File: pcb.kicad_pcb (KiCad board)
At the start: 2 copper layers, 40.6 x 40.6 mm, 3 parts

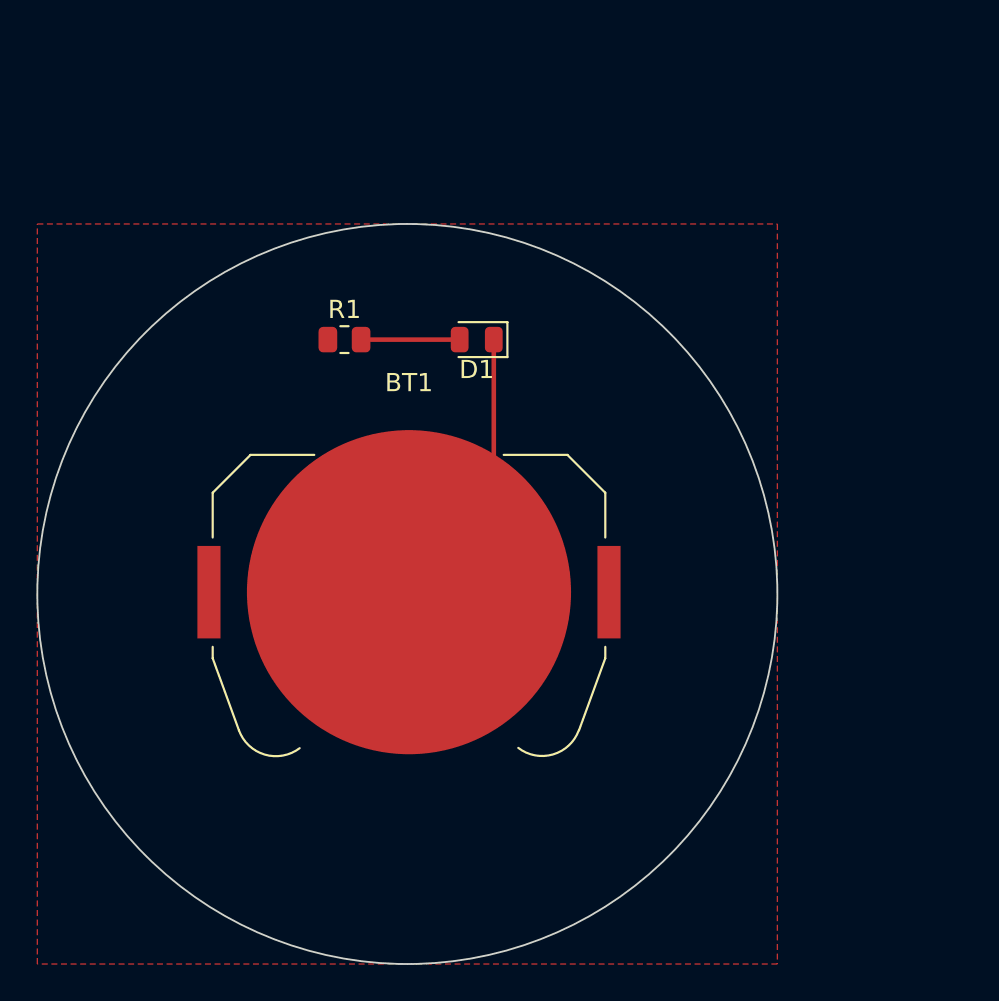
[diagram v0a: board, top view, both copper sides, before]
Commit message: inital layout
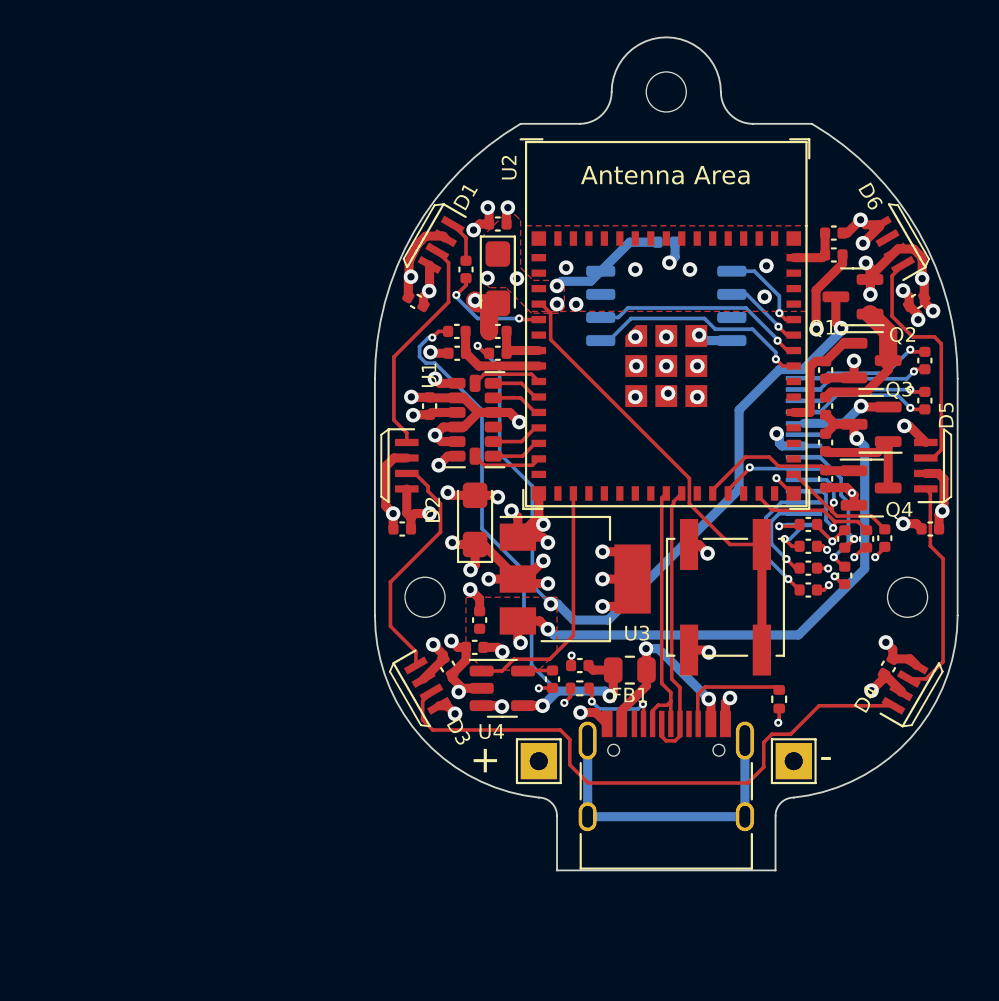
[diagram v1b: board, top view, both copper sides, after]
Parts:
- removed BT1: CR2032, Battery:BatteryHolder_Keystone_3034_1x20mm
- added C1: 100n, Capacitor_SMD:C_0402_1005Metric, F.Cu at (145.2, 67.8)
- added C10: 100n, Capacitor_SMD:C_0402_1005Metric, F.Cu at (146.0, 73.5)
- added C11: 4u7, Capacitor_SMD:C_0402_1005Metric, F.Cu at (154.2, 87.8)
- added C12: 4u7, Capacitor_SMD:C_0402_1005Metric, F.Cu at (168.8, 80.8)
- added C13: 100n, Capacitor_SMD:C_0402_1005Metric, F.Cu at (168.8, 82.8)
- added C14: 1u, Capacitor_SMD:C_0402_1005Metric, F.Cu at (173.2, 73.2)
- added C15: 2u2, Capacitor_SMD:C_0402_1005Metric, F.Cu at (166.8, 82.4)
- added C16: 4u7, Capacitor_SMD:C_0402_1005Metric, F.Cu at (166.8, 81.2)
- added C17: 1u, Capacitor_SMD:C_0402_1005Metric, F.Cu at (173.2, 71.0)
- added C18: 100n, Capacitor_SMD:C_0402_1005Metric, F.Cu at (166.8, 80.0)
- added C19: 1u, Capacitor_SMD:C_0402_1005Metric, F.Cu at (168.2, 64.0)
- added C2: 100n, Capacitor_SMD:C_0402_1005Metric, F.Cu at (144.5, 80.2)
- added C20: 10u tantalum, Capacitor_Tantalum_SMD:CP_EIA-3216-10_Kemet-I, F.Cu at (149.8, 66.5)
- added C21: 100n, Capacitor_SMD:C_0402_1005Metric, F.Cu at (149.8, 63.5)
- added C22: 100n, Capacitor_SMD:C_0402_1005Metric, B.Cu at (159.0, 64.5)
- added C3: 100n, Capacitor_SMD:C_0402_1005Metric, F.Cu at (147.0, 87.8)
- added C4: 100n, Capacitor_SMD:C_0402_1005Metric, F.Cu at (171.2, 87.8)
- added C5: 100n, Capacitor_SMD:C_0402_1005Metric, F.Cu at (173.5, 80.2)
- added C6: 100n, Capacitor_SMD:C_0402_1005Metric, F.Cu at (172.8, 67.8)
- added C7: 10u, Capacitor_SMD:C_0402_1005Metric, F.Cu at (148.8, 85.2)
- added C8: 10u tantalum, Capacitor_Tantalum_SMD:CP_EIA-3216-10_Kemet-I, F.Cu at (148.5, 79.8)
- added C9: 100n, Capacitor_SMD:C_0402_1005Metric, F.Cu at (148.5, 86.8)
- added D2: WS2812B-4020, WS2812B-4020:WS2812B-4020, F.Cu at (144.8, 76.8)
- added D3: WS2812B-4020, WS2812B-4020:WS2812B-4020, F.Cu at (145.9, 88.9)
- added D4: WS2812B-4020, WS2812B-4020:WS2812B-4020, F.Cu at (172.1, 88.9)
- added D5: WS2812B-4020, WS2812B-4020:WS2812B-4020, F.Cu at (173.2, 76.8)
- added D6: WS2812B-4020, WS2812B-4020:WS2812B-4020, F.Cu at (171.4, 64.6)
- added FB1: 100R@100MHz, Resistor_SMD:R_0805_2012Metric, F.Cu at (157.0, 88.0)
- added H1: MountingHole, MountingHole:MountingHole_2.2mm_M2, F.Cu at (172.2, 84.0)
- added H2: MountingHole, MountingHole:MountingHole_2.2mm_M2, F.Cu at (145.8, 84.0)
- added H3: MountingHole, MountingHole:MountingHole_2.2mm_M2, F.Cu at (159.0, 56.2)
- added J1: USB_C_Receptacle_USB2.0, Connector_USB:USB_C_Receptacle_HRO_TYPE-C-31-M-12, F.Cu at (159.0, 95.0)
- added J2: OLED, OLED_FFC:FPC_14, B.Cu at (166.6, 76.0)
- added Q1: 2N7002, Package_TO_SOT_SMD:SOT-23, F.Cu at (170.2, 71.0)
- added Q2: Si2301CDS, Package_TO_SOT_SMD:SOT-23, F.Cu at (169.2, 67.5)
- added Q3: 2N7002, Package_TO_SOT_SMD:SOT-23, F.Cu at (170.2, 78.0)
- added Q4: Si2301CDS, Package_TO_SOT_SMD:SOT-23, F.Cu at (170.2, 74.5)
- added R10: 4k7, Capacitor_SMD:C_0402_1005Metric, F.Cu at (170.0, 80.8)
- added R11: 4k7, Capacitor_SMD:C_0402_1005Metric, F.Cu at (171.0, 80.8)
- added R12: 10k, Capacitor_SMD:C_0402_1005Metric, F.Cu at (168.2, 65.2)
- added R15: 100k, Capacitor_SMD:C_0402_1005Metric, F.Cu at (149.8, 70.6)
- added R16: 100k, Capacitor_SMD:C_0402_1005Metric, F.Cu at (149.8, 69.4)
- added R17: 100k, Capacitor_SMD:C_0402_1005Metric, F.Cu at (147.5, 69.4)
- added R18: 100k, Capacitor_SMD:C_0402_1005Metric, F.Cu at (147.5, 70.6)
- added R2: 10k, Capacitor_SMD:C_0402_1005Metric, F.Cu at (167.8, 73.5)
- added R3: 10k, Capacitor_SMD:C_0402_1005Metric, F.Cu at (167.8, 77.5)
- added R4: 100, Capacitor_SMD:C_0402_1005Metric, F.Cu at (148.0, 66.0)
- added R5: 10k, Capacitor_SMD:C_0402_1005Metric, F.Cu at (152.8, 88.5)
- added R6: 5k1, Resistor_SMD:R_0402_1005Metric, F.Cu at (154.2, 89.0)
- added R7: 5k1, Resistor_SMD:R_0402_1005Metric, F.Cu at (165.2, 89.6)
- added R8: 10k, Capacitor_SMD:C_0402_1005Metric, F.Cu at (167.8, 75.5)
- added R9: 560k, Capacitor_SMD:C_0402_1005Metric, F.Cu at (166.8, 83.6)
- added SW1: SW_Push, Button_Switch_SMD:SW_Push_1P1T_NO_CK_KSC7xxJ, F.Cu at (162.2, 84.0)
- added TP1: Batt+, TestPoint:TestPoint_THTPad_2.0x2.0mm_Drill1.0mm, F.Cu at (152.0, 93.0)
- added TP2: Batt-, TestPoint:TestPoint_THTPad_2.0x2.0mm_Drill1.0mm, F.Cu at (166.0, 93.0)
- added U1: ADXL375, Package_LGA:LGA-14_3x5mm_P0.8mm_LayoutBorder1x6y, F.Cu at (148.5, 74.2)
- added U2: ESP32-S3-MINI-1, PCM_Espressif:ESP32-S2-MINI-1, F.Cu at (159.0, 71.3)
- added U3: AMS1117-3.3, Package_TO_SOT_SMD:SOT-223-3_TabPin2, F.Cu at (154.0, 83.0)
- added U4: MCP73831-2-OT, Package_TO_SOT_SMD:SOT-23-5, F.Cu at (150.0, 89.0)
- added U5: W25Q128JVS, Package_SO:SOIC-8_5.23x5.23mm_P1.27mm, B.Cu at (159.0, 68.0)
- D1: value LED -> WS2812B-4020; footprint LED_SMD:LED_0805_2012Metric -> WS2812B-4020:WS2812B-4020
- R1: value 1k -> 10k; footprint Resistor_SMD:R_0805_2012Metric -> Capacitor_SMD:C_0402_1005Metric
- moved R1 26.5 mm to (167.8, 71.5), turned to -90 degrees
- moved D1 5.56 mm to (146.6, 64.6), turned to 60 degrees
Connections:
- D1 pad 1: GND -> Net-(D1-DIN)
- D1 pad 2: Net-(D1-A) -> /LEDs/VLED
- R1 pad 1: Net-(BT1-+) -> LED_EN
- R1 pad 2: Net-(D1-A) -> GND
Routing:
- net VBAT: track 0.00 -> 86.6 mm, vias 0 -> 8
- net GND: track 15.6 -> 78.2 mm, vias 0 -> 58
- net +3.3V: track 0.00 -> 46.1 mm, vias 0 -> 21
- net USB_VBUS: track 0.00 -> 32.4 mm, vias 0 -> 3
- net Net-(D3-DOUT): track 0.00 -> 32.4 mm
- net /LEDs/VLED: track 0.00 -> 27.8 mm, vias 0 -> 9
- net /BOOT: track 0.00 -> 25.2 mm
- net unconnected-(J1-SHIELD-PadS1): track 0.00 -> 17.0 mm
- net USB_D+: track 0.00 -> 15.6 mm
- net USB_D-: track 0.00 -> 14.9 mm
- net CHARGE_STAT: track 0.00 -> 13.6 mm
- net Net-(D2-DOUT): track 0.00 -> 13.3 mm
- net Net-(D5-DOUT): track 0.00 -> 13.3 mm
- net FLASH-SDI: track 0.00 -> 12.4 mm, vias 0 -> 1
- net Net-(D1-DOUT): track 0.00 -> 12.3 mm
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- added copper zone on F.Cu, net +3.3V
- added copper zone on In2.Cu, net +3.3V
- added copper zone on In2.Cu, net /LEDs/VLED
- added copper zone on F.Cu, net GND
- added copper zone on In1.Cu, net GND
- added copper zone on F.Cu, net VBAT
- added copper zone on In2.Cu, net VBAT
- removed copper zone on F.Cu, net Net-(BT1-+)
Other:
- board size 40.6 x 40.6 mm -> 32 x 45.8 mm
- copper layers 2 -> 4
- board text added: "+"
- board text added: "-"
- board text added: "-OLED-"
- board text added: "EGGSHELLEROMETER Rev. 0.1"
- board text added: "Jack LeFevre July 2023"
